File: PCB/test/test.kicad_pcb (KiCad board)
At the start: 2 copper layers, 47.3 x 33.1 mm, 60 parts, among them CN4 HEADER_1X4, CN5 UFL, SW2 MLL1200S_TE, U1 STM32WBxx_QFN48, U2 USBLC6-2SC6, U3 LD3985M33R, X1 NX2016_32MHz, X2 NX2012_32K768Hz

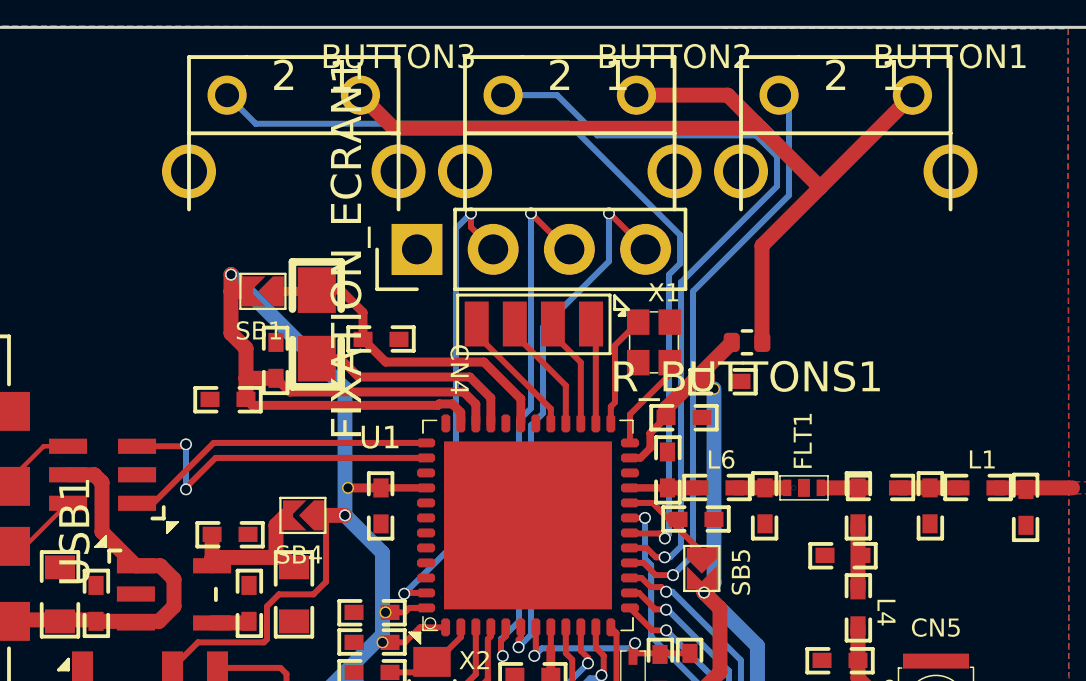
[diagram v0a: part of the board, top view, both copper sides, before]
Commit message: fix d'une erreur
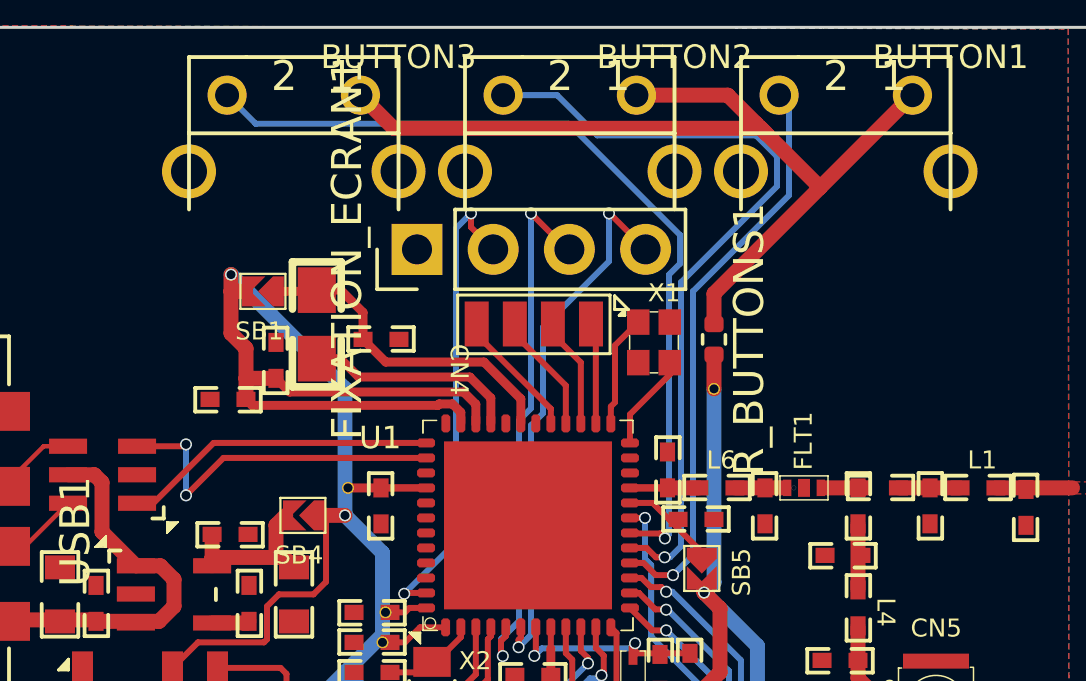
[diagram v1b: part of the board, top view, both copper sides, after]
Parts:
- removed C1: 100nF, Library:0402_CAP_NPOL
- removed C2: 100pF, Library:0402_CAP_NPOL
- moved R_BUTTONS1 1.10 mm to (141.2, 86.9), turned to -90 degrees
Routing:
- net 3V3: track 113.4 -> 109.1 mm
